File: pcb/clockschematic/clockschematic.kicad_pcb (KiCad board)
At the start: 2 copper layers, 121.9 x 96.5 mm, 19 parts, among them SW1 SW_Push, SW2 SW_Push, SW3 SW_Push, SW4 SW_Push, U0 RPi_Pico_TH, U1 RDA5807M_Module, U2 LM386, U3 LM386

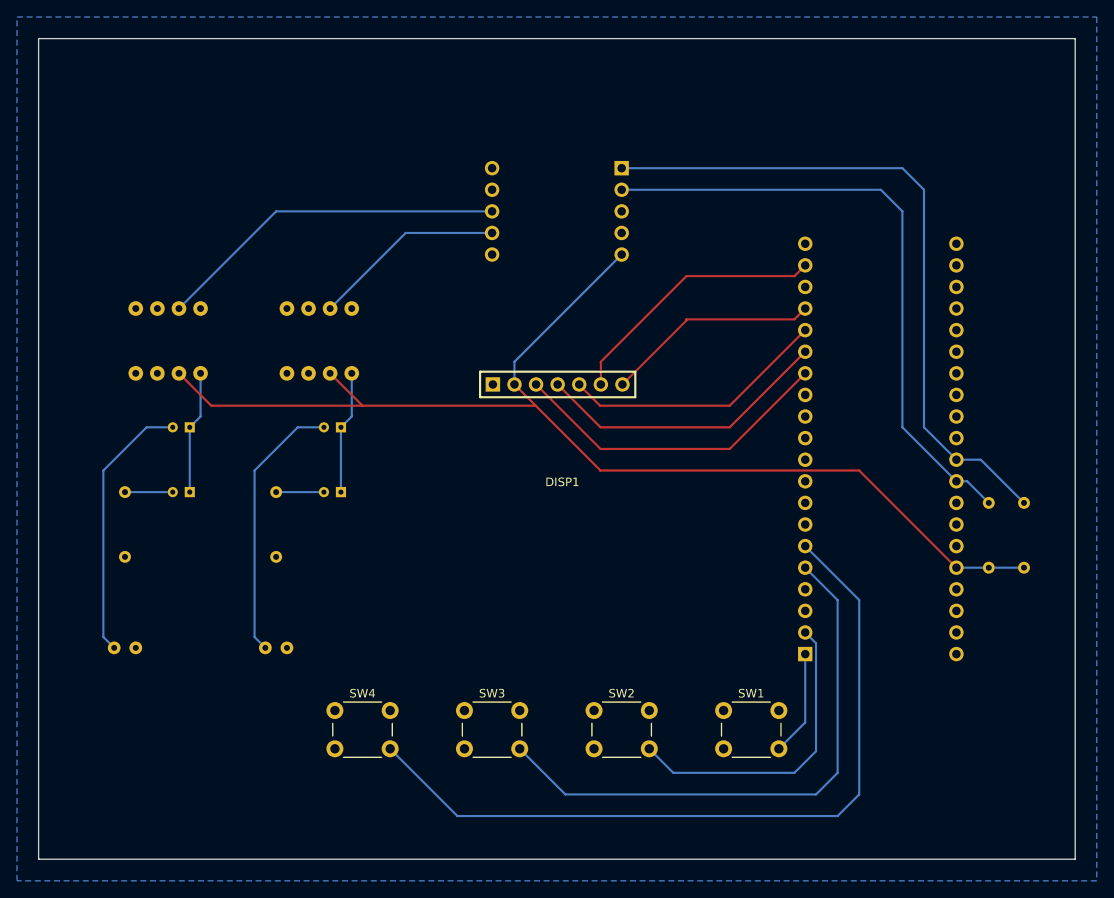
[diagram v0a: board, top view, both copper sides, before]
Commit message: update
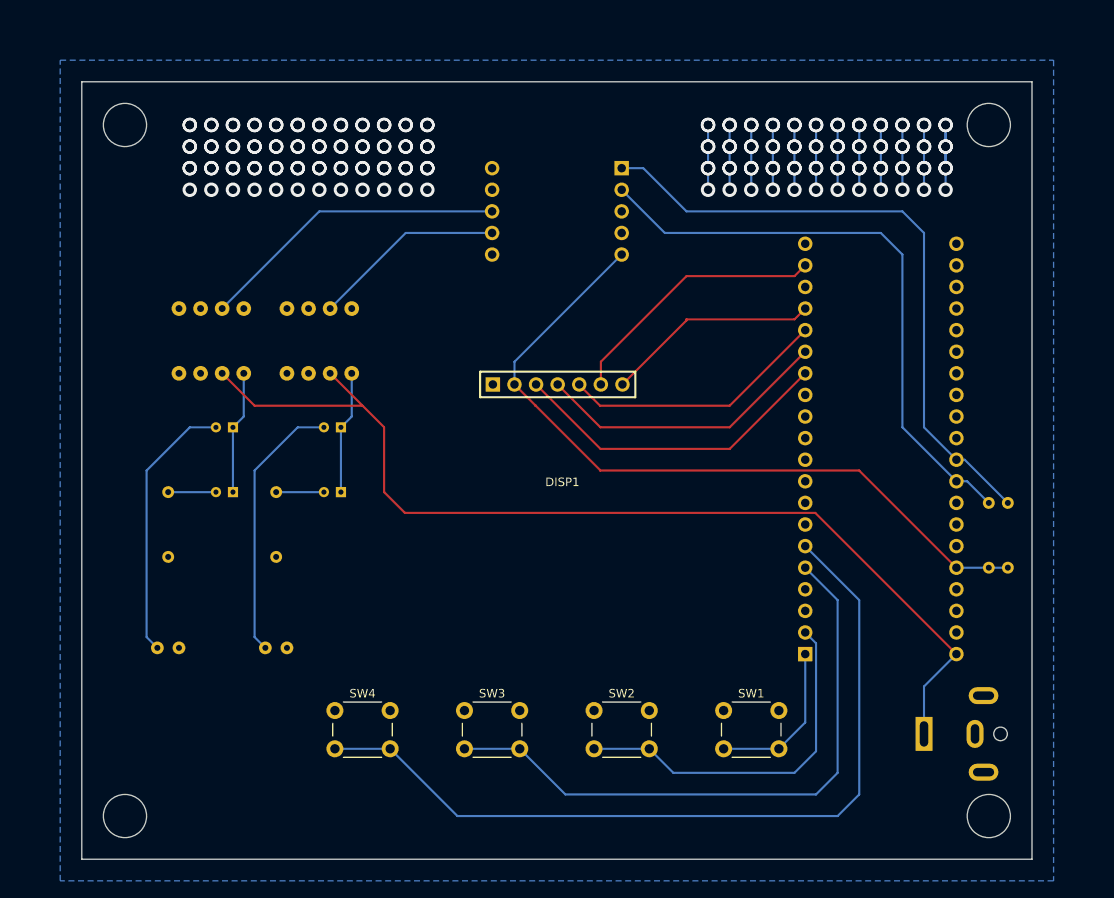
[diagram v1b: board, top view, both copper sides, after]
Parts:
- added J1: Barrel_Jack, Connector_BarrelJack:BarrelJack_CUI_PJ-063AH_Horizontal, B.Cu at (190.5, 102.1)
- moved U2 5.08 mm to (106.7, 55.9)
- moved C1 5.08 mm to (109.2, 66.0)
- moved C2 5.08 mm to (109.2, 73.7)
- moved LS1 5.08 mm to (101.6, 94.0)
- moved R3 5.08 mm to (101.6, 73.7)
- moved R1 1.90 mm to (200.4, 82.5)
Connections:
- U0 pad 40: unconnected-(U0-Pad40) -> +5V
- U2 pad 6: +3.3V -> +5V
- U3 pad 6: +3.3V -> +5V
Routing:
- net +5V: track 0.00 -> 120.9 mm
- net (no net): track 0.00 -> 96.5 mm, vias 0 -> 168
- net +3.3V: track 138.3 -> 87.5 mm
- net Net-(SW4-Pad2): track 91.3 -> 97.8 mm
- net Net-(SW3-Pad2): track 66.4 -> 72.9 mm
- net Net-(SW2-Pad2): track 36.3 -> 42.8 mm
- net Net-(SW1-Pad2): track 12.4 -> 18.9 mm
- net Net-(U1-Pad8): track 41.6 -> 36.5 mm
- net Net-(R1-Pad2): track 80.0 -> 75.1 mm
- net Net-(R2-Pad2): track 73.3 -> 70.3 mm
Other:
- board size 121.9 x 96.5 mm -> 111.8 x 91.4 mm
